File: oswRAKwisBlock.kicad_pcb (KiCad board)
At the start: 4 copper layers, 33.8 x 46 mm, 69 parts, among them J1 WisBlock, J2 0524352471, J4 10114830-10102LF, J5 USB micro, Q1 SI1308EDL-T1-GE3, U1 MCP73811T-420I/OT, U2 MAX2769B, U3 MAX8510EXK29+T, U4 MAX8510EXK29+T, U5 MIC5365-3.0YC5-TR, Y1 TXETCDSANF-16.368000

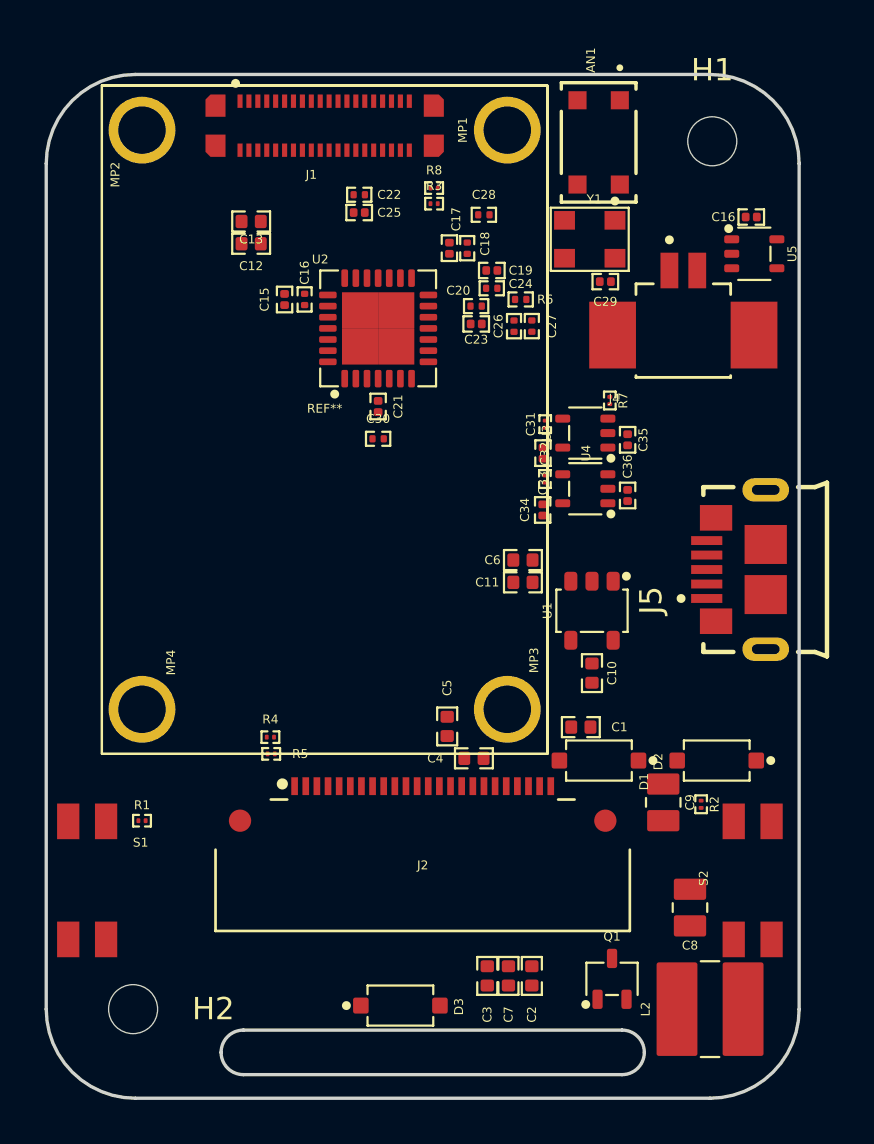
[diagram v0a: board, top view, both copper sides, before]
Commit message: working on the layout some.
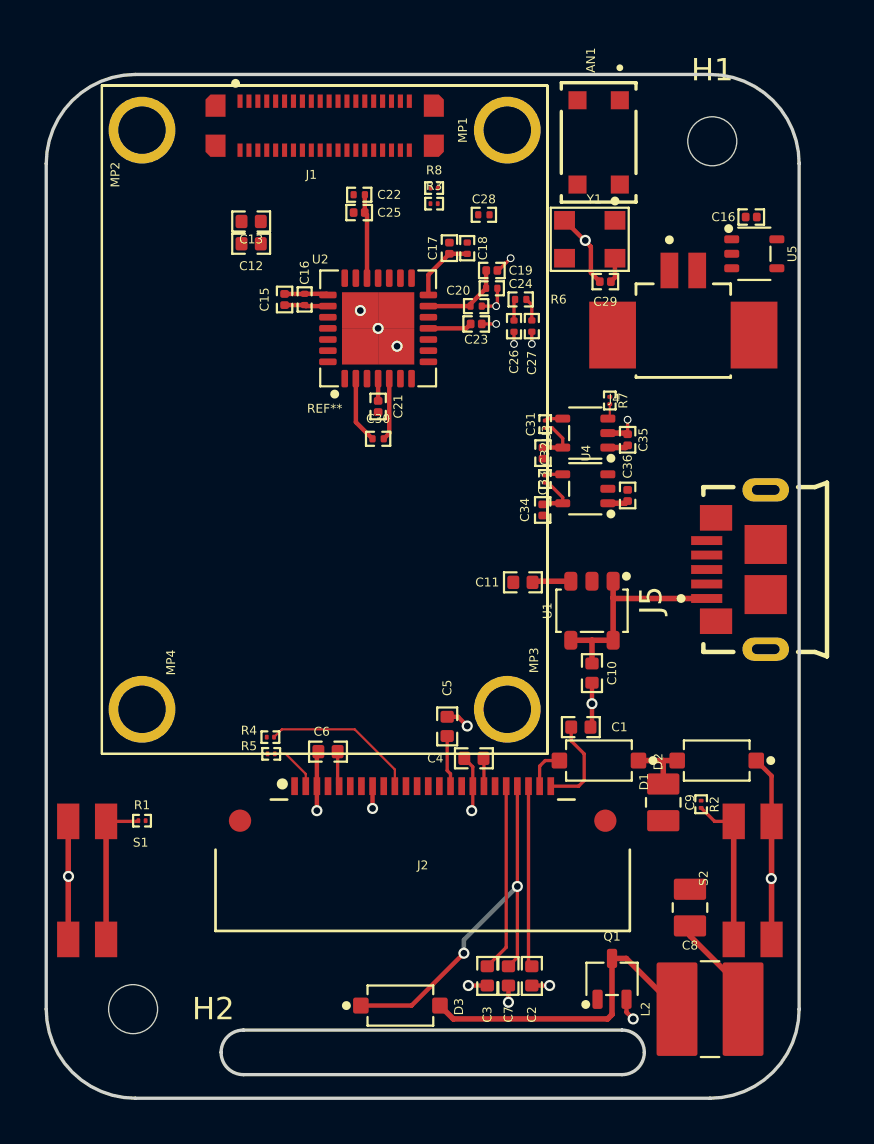
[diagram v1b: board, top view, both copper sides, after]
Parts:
- moved C6 12.3 mm to (132.5, 130.4)
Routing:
- net GND: track 0.00 -> 37.3 mm, vias 0 -> 21
- net /PREVGH: track 0.00 -> 17.8 mm, vias 0 -> 2
- net Net-(Q1-D): track 0.00 -> 14.4 mm
- net VDD_GPS_A: track 0.00 -> 11.0 mm
- net VDD_GPS_B: track 0.00 -> 10.2 mm
- net VUSB_BUS: track 0.00 -> 9.80 mm
- net VDD: track 0.00 -> 8.89 mm
- net Net-(J2-Pin_20): track 0.00 -> 8.44 mm
- net Net-(J2-Pin_22): track 0.00 -> 8.15 mm
- net /RES: track 0.00 -> 7.06 mm
- net /BTN2: track 0.00 -> 7.01 mm
- net /BTN1: track 0.00 -> 6.76 mm
- net Net-(J2-Pin_24): track 0.00 -> 4.24 mm
- net Net-(U2-LNAOUT): track 0.00 -> 3.01 mm
- net Net-(U2-MIXIN): track 0.00 -> 2.80 mm
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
